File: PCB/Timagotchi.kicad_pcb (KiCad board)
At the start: 2 copper layers, 9 parts, among them J1 Conn_01x04, SW1 SW_Omron_B3FS, SW2 SW_Omron_B3FS, SW3 SW_Omron_B3FS, U1 XIAO-ESP32-S3-Plus-SMD, U2 MAX98357A

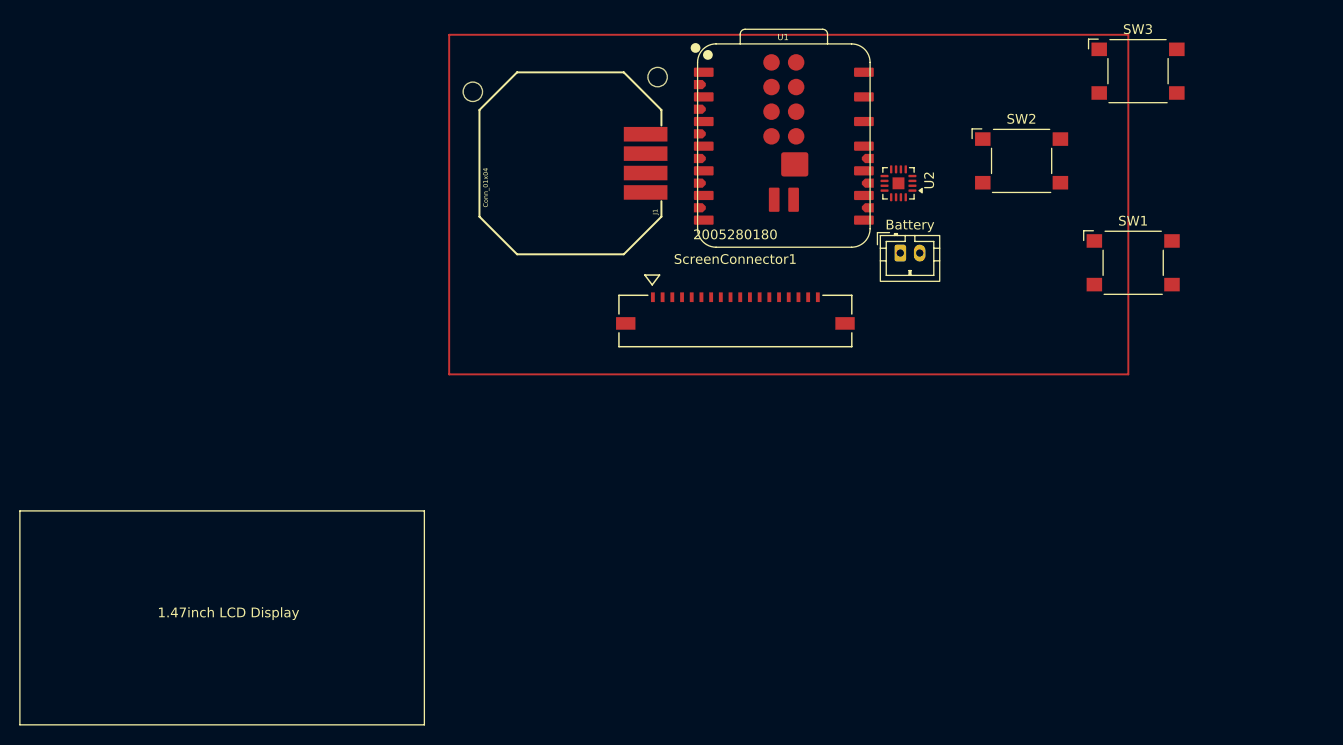
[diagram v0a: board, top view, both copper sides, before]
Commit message: puh cuh buh 2
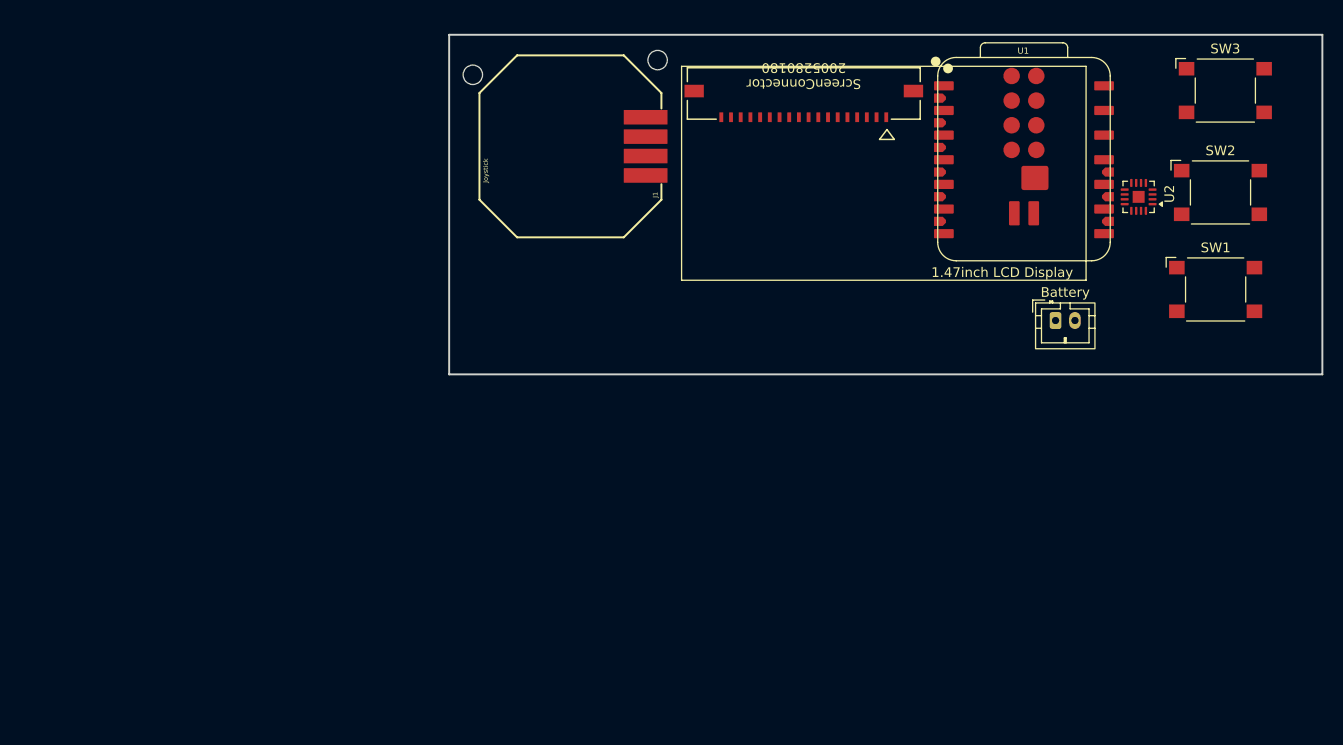
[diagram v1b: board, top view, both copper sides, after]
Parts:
- J1: value Conn_01x04 -> Joystick
- moved 1.47inch LCD Display 82.2 mm to (149.0, 41.8)
- moved U1 24.8 mm to (184.2, 51.4)
- moved U2 24.8 mm to (196.1, 55.2)
- moved ScreenConnector 24.5 mm to (161.5, 44.5), turned to 180 degrees
- moved SW2 20.8 mm to (204.5, 54.8)
- moved Battery 17.4 mm to (187.5, 68.0)
- moved SW3 9.22 mm to (205.0, 44.2)
- moved SW1 8.93 mm to (204.0, 64.8)
- moved J1 1.75 mm to (137.5, 50.0)
- renumbered ScreenConnector1 to ScreenConnector
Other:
- board outline added: 90 x 35 mm

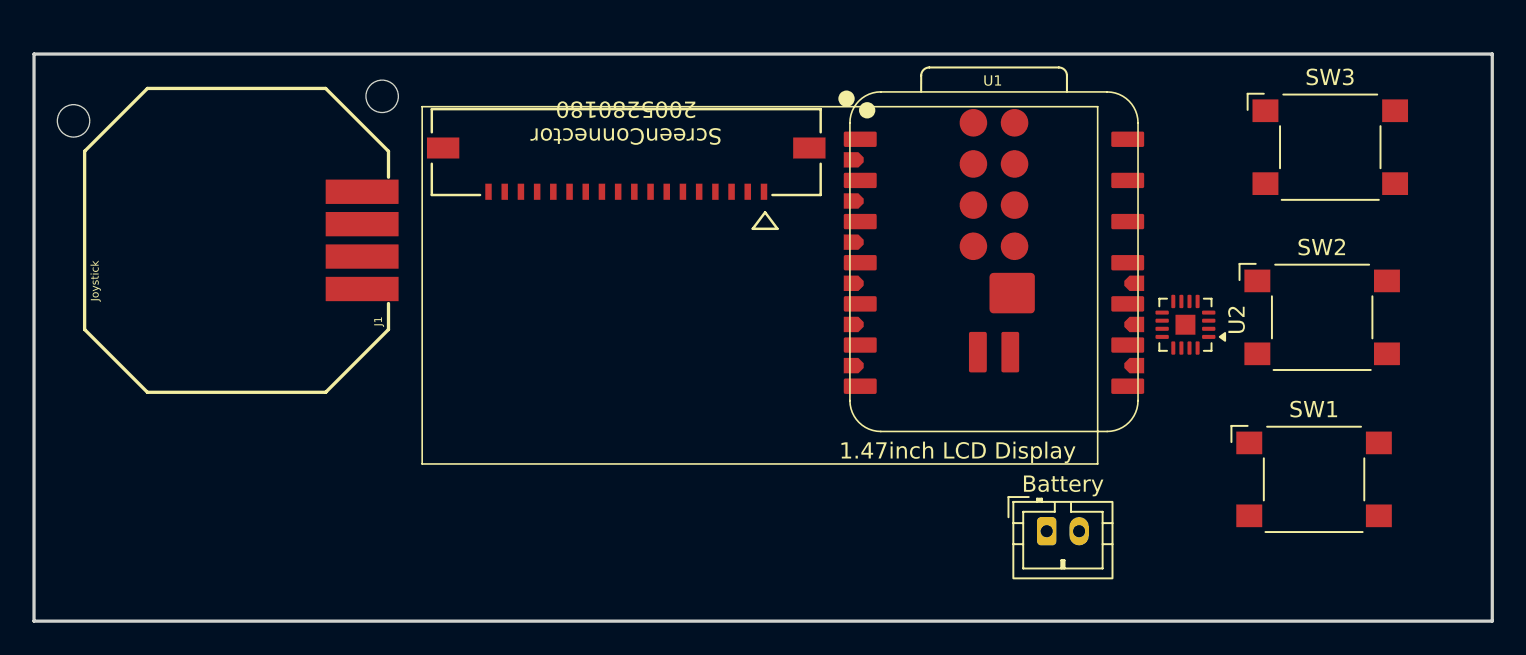
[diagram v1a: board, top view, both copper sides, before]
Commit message: PCB wiringgg
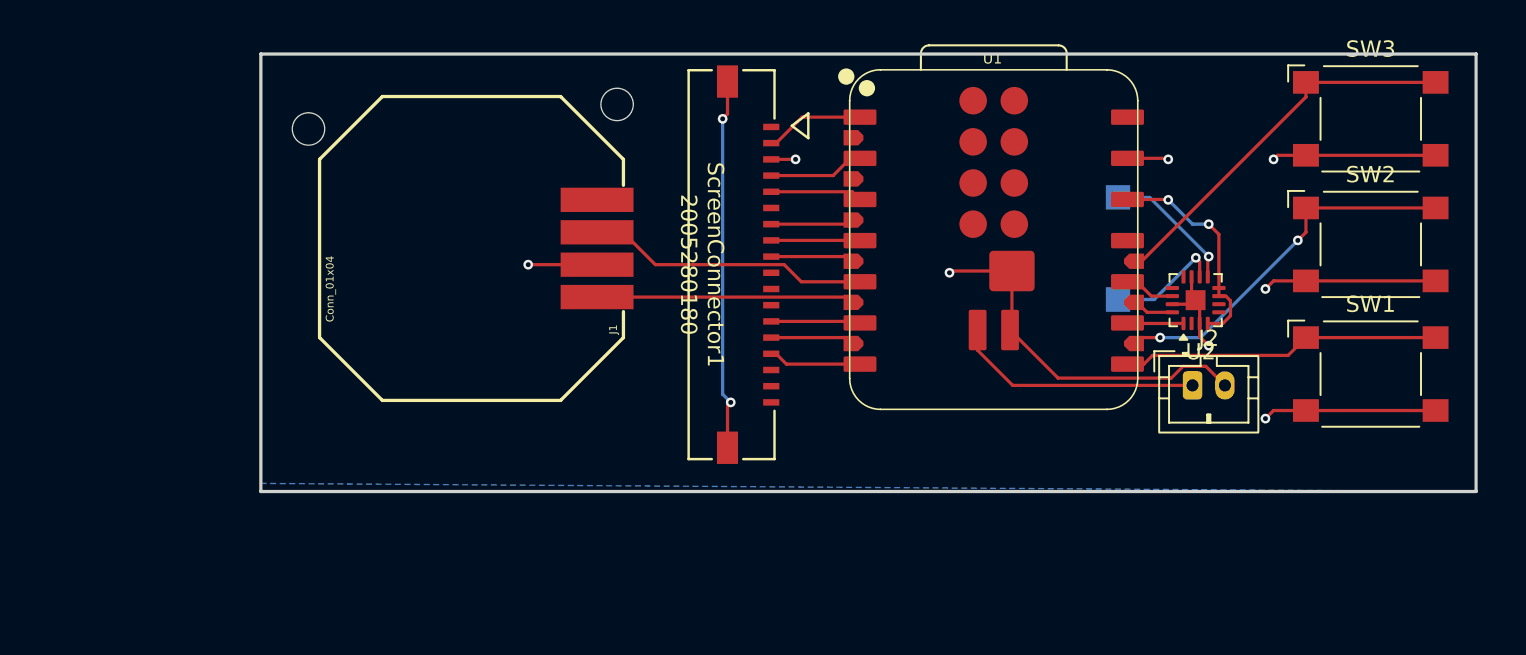
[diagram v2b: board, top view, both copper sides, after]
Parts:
- removed 1.47inch LCD Display: 1.47inch LCD Display, Library:1.47inch LCD Display
- added LS1: CMS-201438-058S, Speaker speaker:SPKR_CMS-201438-058S, B.Cu at (185.5, 50.5)
- J1: value Joystick -> Conn_01x04
- moved J1 14.5 mm to (152.0, 50.5)
- moved J2 12.7 mm to (196.5, 59.0)
- moved ScreenConnector1 9.52 mm to (168.1, 51.5), turned to -90 degrees
- moved SW1 7.38 mm to (207.5, 58.2)
- moved SW2 5.41 mm to (207.5, 50.2)
- moved SW3 3.05 mm to (207.5, 42.5)
- moved U2 1.64 mm to (196.7, 53.7), turned to 90 degrees
- moved U1 1.36 mm to (184.2, 50.0)
- renumbered Battery to J2, ScreenConnector to ScreenConnector1
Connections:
- ScreenConnector1 pad 15: /TP_INT -> /LCD_DC
- ScreenConnector1 pad 7: /LCD_DC -> /TP_INT
- U1 pad 1: /TP_INT -> /LCD_BL
- U1 pad 10: /I2S_SD -> /I2S_WS
- U1 pad 17: /SCLK -> /TP_INT
- U1 pad 19: /VPOS -> /HPOS
- U1 pad 2: /MOSI -> /SCLK
- U1 pad 20: /HPOS -> /TP_SDA
- U1 pad 3: /LCD_BL -> /MOSI
- U1 pad 5: /TP_SDA -> /VPOS
- U1 pad 9: /I2S_WS -> /I2S_SD
- U2 pad 10: unconnected-(U2-OUTN-Pad10) -> Net-(U2-OUTN)
- U2 pad 9: unconnected-(U2-OUTP-Pad9) -> Net-(U2-OUTP)
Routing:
- net GND: track 0.00 -> 91.9 mm, vias 0 -> 10
- net /SW3: track 0.00 -> 23.7 mm
- net /SW2: track 0.00 -> 23.0 mm, vias 0 -> 2
- net /SW1: track 0.00 -> 19.7 mm
- net /VPOS: track 0.00 -> 17.5 mm
- net /HPOS: track 0.00 -> 16.0 mm
- net /VBAT: track 0.00 -> 15.4 mm
- net +3.3V: track 0.00 -> 13.7 mm, vias 0 -> 2
- net Net-(U2-OUTP): track 0.00 -> 8.39 mm, vias 0 -> 1
- net Net-(U2-OUTN): track 0.00 -> 7.14 mm, vias 0 -> 1
- net /LCD_BL: track 0.00 -> 6.14 mm
- net /SCLK: track 0.00 -> 5.92 mm
- net /LCD_DC: track 0.00 -> 5.74 mm
- net /MOSI: track 0.00 -> 5.67 mm
- net /TP_SCL: track 0.00 -> 5.51 mm
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- added copper zone on F.Cu, net +3.3V
- added copper zone on B.Cu, net GND
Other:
- board size 90 x 35 mm -> 75 x 27 mm
